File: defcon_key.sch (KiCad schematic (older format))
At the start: 12 parts, among them U1 ATTINY84-20PU

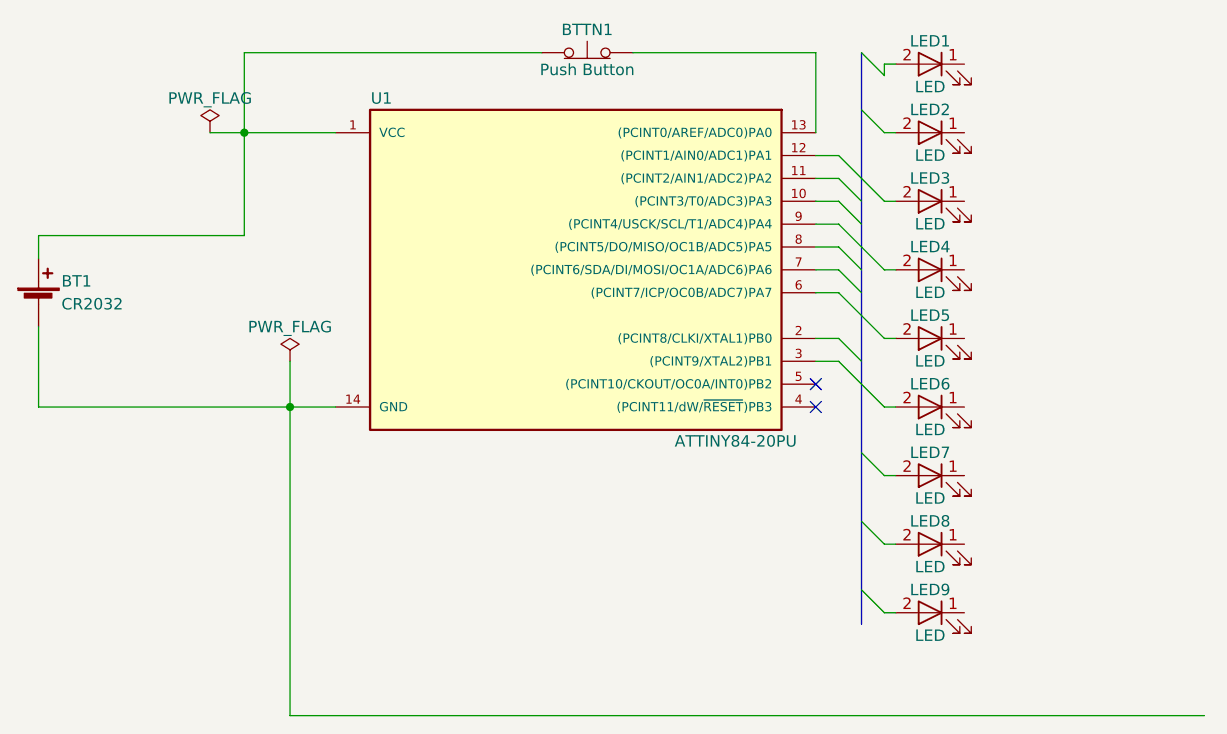
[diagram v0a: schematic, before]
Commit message: IMPROVEMENTS!
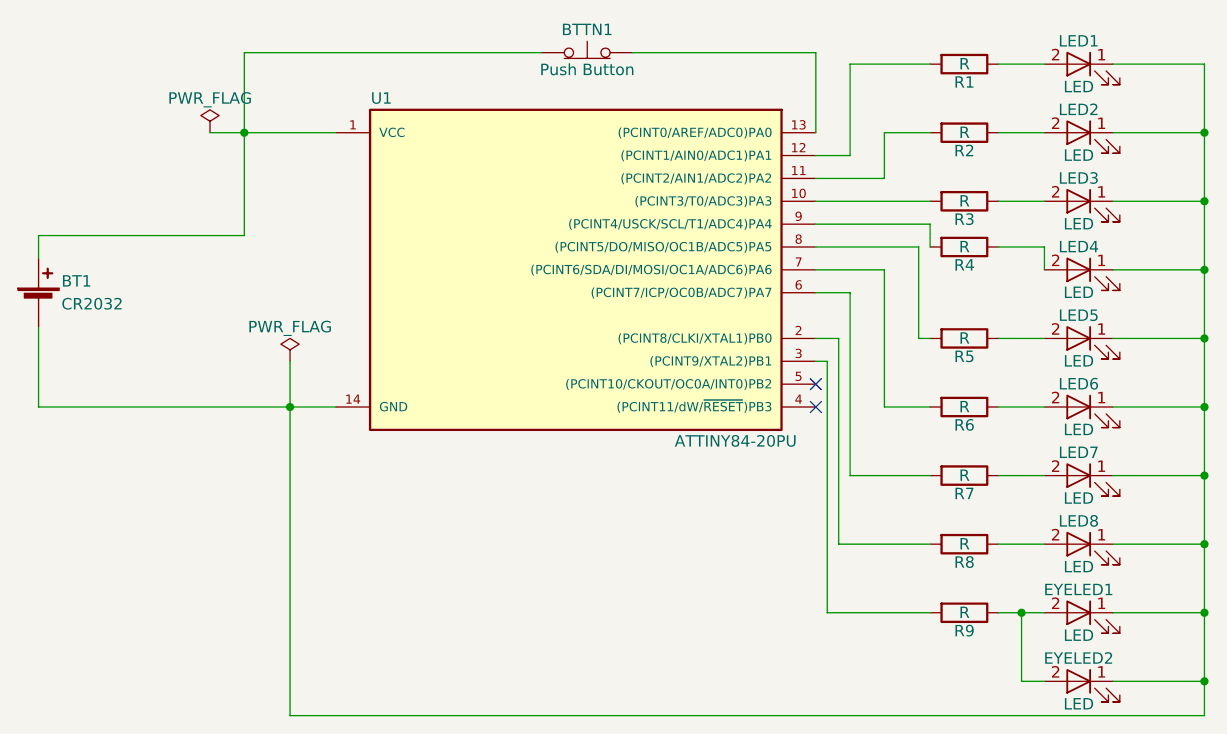
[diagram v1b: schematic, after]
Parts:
- added EYELED2: LED, LEDs:LED_D5.0mm, symbol LED
- added R1, R2, R3, R4, R5, R6, R7, R8, R9: R, Resistors_THT:R_Axial_DIN0207_L6.3mm_D2.5mm_P7.62mm_Horizontal, symbol R
- BT1: footprint (none) -> Battery_Holders:Keystone_103_1x20mm-CoinCell
- BTTN1: footprint (none) -> Buttons_Switches_THT:SW_PUSH-12mm
- EYELED1: renamed from LED9; footprint (none) -> LEDs:LED_D5.0mm
- LED1, LED2, LED3, LED4, LED5, LED6, LED7, LED8: footprint (none) -> LEDs:LED_D5.0mm
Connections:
- net at U1.10 ((PCINT3/T0/ADC3)PA3): now also R3.2
- net at U1.11 ((PCINT2/AIN1/ADC2)PA2): now also R2.2
- net at U1.12 ((PCINT1/AIN0/ADC1)PA1): now also R1.2
- net at BT1.2 (-), U1.14 (GND): now also EYELED1.1 (K), LED1.1 (K), LED2.1 (K), LED3.1 (K), LED4.1 (K), LED5.1 (K), LED6.1 (K), LED7.1 (K), LED8.1 (K), EYELED2.1 (K)
- net at U1.2 ((PCINT8/CLKI/XTAL1)PB0): now also R8.2
- net at U1.3 ((PCINT9/XTAL2)PB1): now also R9.2
- net at U1.6 ((PCINT7/ICP/OC0B/ADC7)PA7): now also R7.2
- net at U1.7 ((PCINT6/SDA/DI/MOSI/OC1A/ADC6)PA6): now also R6.2
- net at U1.8 ((PCINT5/DO/MISO/OC1B/ADC5)PA5): now also R5.2
- net at U1.9 ((PCINT4/USCK/SCL/T1/ADC4)PA4): now also R4.2
- net at LED2.2 (A): now also R2.1
- net at LED3.2 (A): now also R3.1
- net at LED4.2 (A): now also R4.1
- net at LED5.2 (A): now also R5.1
- net at LED6.2 (A): now also R6.1
- net at LED7.2 (A): now also R7.1
- net at LED1.2 (A): now also R1.1
- net at LED8.2 (A): now also R8.1
- net at EYELED1.2 (A): now also EYELED2.2 (A), R9.1
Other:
- moved on the sheet: EYELED1, LED1, LED2, LED3, LED4, LED5, LED6, LED7, LED8
